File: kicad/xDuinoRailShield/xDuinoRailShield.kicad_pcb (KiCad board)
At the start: 2 copper layers, 63.5 x 53.3 mm, 40 parts, among them J501 Screw_Terminal_01x02, Q301 T2N7002BK, Q401 S8050, Q402 S8550, Q403 S8550, Q404 S8050, U201 TPS5430DDA, U301 6N137, U302 EL817

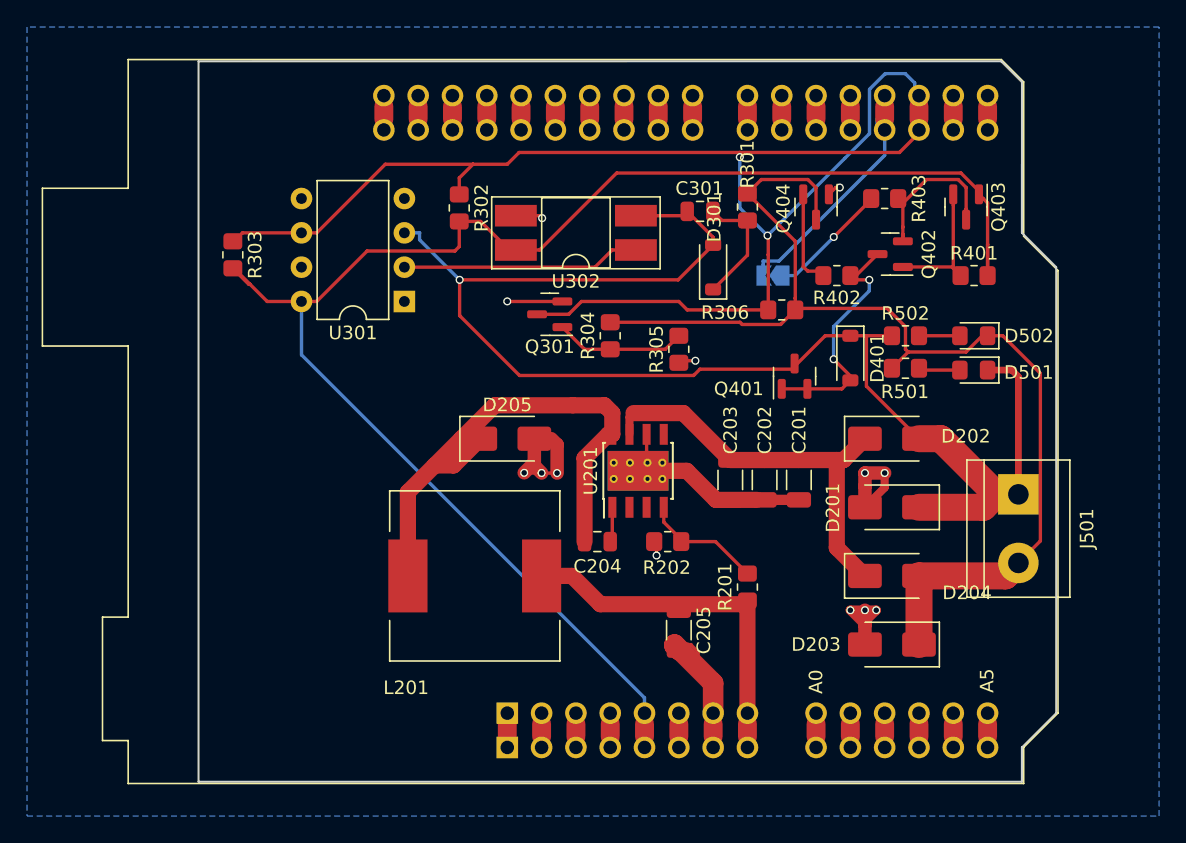
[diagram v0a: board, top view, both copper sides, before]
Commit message: xXiaoCentralMini
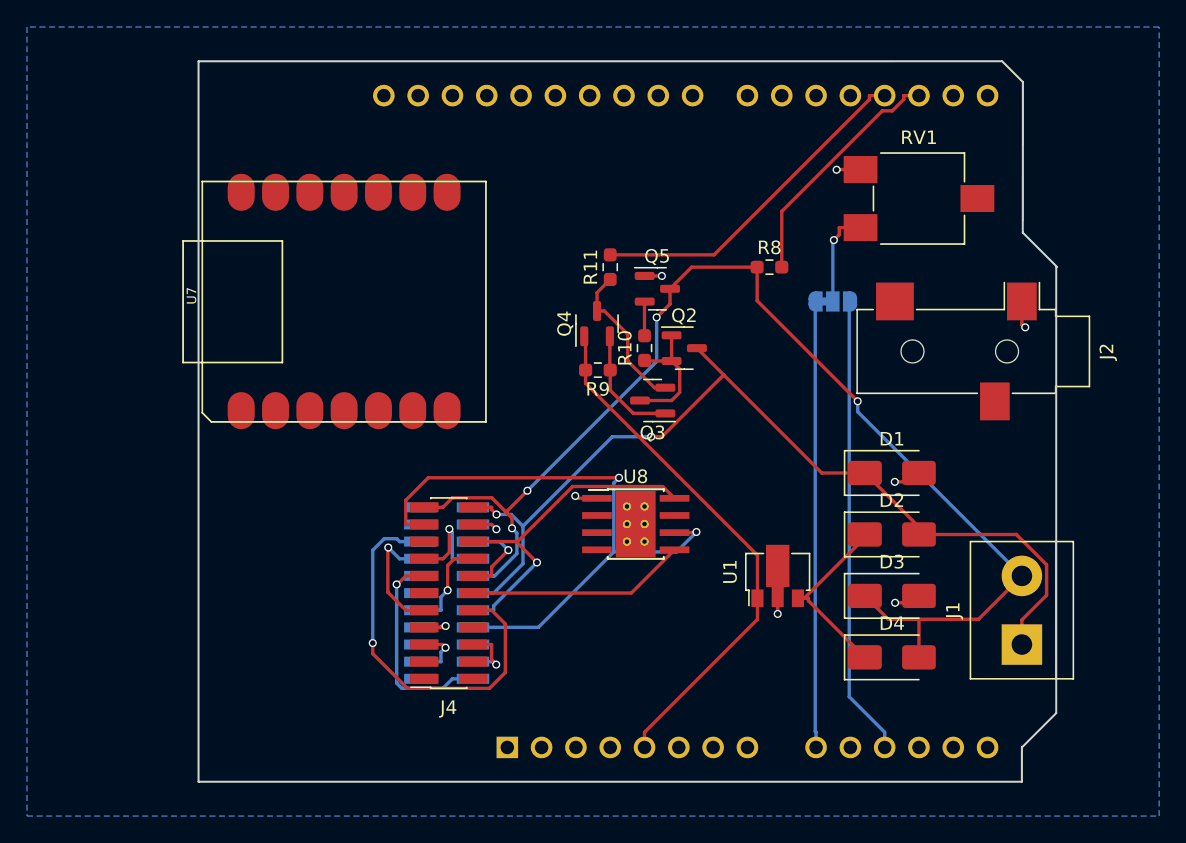
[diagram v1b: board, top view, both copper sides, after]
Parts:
- removed A501: Arduino_UNO_R3, Olis_Footprints:Arduino_UNO_R3_Double_Rows
- removed C201, C202, C203, C205: 10uF, Capacitor_SMD:C_1206_3216Metric
- removed C204: 10nF, Capacitor_SMD:C_0805_2012Metric
- removed C301: 1nF, Capacitor_SMD:C_0805_2012Metric
- removed D201, D202, D203, D204, D205: SS54, Diode_SMD:D_SMA
- removed D301, D401: 1N4148W, Diode_SMD:D_SOD-123
- removed D501, D502: LED, LED_SMD:LED_0805_2012Metric_Pad1.15x1.40mm_HandSolder
- removed J501: Screw_Terminal_01x02, TerminalBlock:TerminalBlock_bornier-2_P5.08mm
- removed JP_RAILCOM401: SolderJumper_2_Open, Jumper:SolderJumper-2_P1.3mm_Open_TrianglePad1.0x1.5mm
- removed L201: 22uH, Inductor_SMD:L_12x12mm_H8mm
- removed Q301: T2N7002BK, Package_TO_SOT_SMD:SOT-23
- removed Q401, Q404: S8050, Package_TO_SOT_SMD:SOT-23
- removed Q402, Q403: S8550, Package_TO_SOT_SMD:SOT-23
- removed R201, R403: 10k, Resistor_SMD:R_0805_2012Metric_Pad1.20x1.40mm_HandSolder
- removed R202: 1.58k, Resistor_SMD:R_0805_2012Metric_Pad1.20x1.40mm_HandSolder
- removed R301: 1k3, Resistor_SMD:R_0805_2012Metric_Pad1.20x1.40mm_HandSolder
- removed R302: 220R, Resistor_SMD:R_0805_2012Metric_Pad1.20x1.40mm_HandSolder
- removed R303: 5k, Resistor_SMD:R_0805_2012Metric_Pad1.20x1.40mm_HandSolder
- removed R304, R305, R402: 6k8, Resistor_SMD:R_0805_2012Metric_Pad1.20x1.40mm_HandSolder
- removed R306: 22k, Resistor_SMD:R_0805_2012Metric_Pad1.20x1.40mm_HandSolder
- removed R401: 20, Resistor_SMD:R_0805_2012Metric_Pad1.20x1.40mm_HandSolder
- removed R501, R502: 3k3, Resistor_SMD:R_0805_2012Metric_Pad1.20x1.40mm_HandSolder
- removed U201: TPS5430DDA, Package_SO:TI_SO-PowerPAD-8_ThermalVias
- removed U301: 6N137, Package_DIP:DIP-8_W7.62mm
- removed U302: EL817, Package_DIP:DIP-4_W8.89mm_SMDSocket_LongPads
- added A1: Arduino_UNO_R3, Module:Arduino_UNO_R3, B.Cu at (125.4, 92.4)
- added D1: SS54, Diode_SMD:D_SMA, F.Cu at (153.9, 72.1)
- added D2: SS54, Diode_SMD:D_SMA, F.Cu at (153.9, 76.6)
- added D3: SS54, Diode_SMD:D_SMA, F.Cu at (153.9, 81.2)
- added D4: SS54, Diode_SMD:D_SMA, F.Cu at (153.9, 85.7)
- added J1: Screw_Terminal_01x02, TerminalBlock:TerminalBlock_bornier-2_P5.08mm, F.Cu at (163.5, 84.8)
- added J2: AudioJack2_Ground, Connector_Audio:Jack_3.5mm_CUI_SJ-3523-SMT_Horizontal, F.Cu at (159.9, 63.1)
- added J3: PLUXX22, Connector_PinHeader_1.27mm:PinHeader_2x11_P1.27mm_Vertical_SMD, B.Cu at (120.9, 81.0)
- added J4: 21mtc, Connector_PinSocket_1.27mm:PinSocket_2x11_P1.27mm_Vertical_SMD, F.Cu at (121.1, 81.0)
- added JP1: DAC_OUTPUT_SELECT, Jumper:SolderJumper-3_P1.3mm_Bridged12_RoundedPad1.0x1.5mm, B.Cu at (149.5, 59.4)
- added Q2: S8050, Package_TO_SOT_SMD:SOT-23, F.Cu at (138.5, 62.8)
- added Q3: S8550, Package_TO_SOT_SMD:SOT-23, F.Cu at (136.2, 66.7)
- added Q4: S8550, Package_TO_SOT_SMD:SOT-23, F.Cu at (132.0, 61.0)
- added Q5: S8050, Package_TO_SOT_SMD:SOT-23, F.Cu at (136.5, 58.4)
- added R10: 6k8, Resistor_SMD:R_0603_1608Metric_Pad0.98x0.95mm_HandSolder, F.Cu at (135.6, 62.8)
- added R11: 10k, Resistor_SMD:R_0603_1608Metric_Pad0.98x0.95mm_HandSolder, F.Cu at (133.0, 56.8)
- added R8: 22k, Resistor_SMD:R_0603_1608Metric_Pad0.98x0.95mm_HandSolder, F.Cu at (144.8, 56.8)
- added R9: 20, Resistor_SMD:R_0603_1608Metric_Pad0.98x0.95mm_HandSolder, F.Cu at (132.1, 64.4)
- added RV1: 10K, Potentiometer_SMD:Potentiometer_ACP_CA6-VSMD_Vertical, F.Cu at (155.9, 51.7)
- added U1: L78L05_SOT89, Package_TO_SOT_SMD:SOT-89-3, F.Cu at (145.4, 79.4)
- added U7: MOUDLE-SEEEDUINO-XIAO-ESP32C3, xiao ESP32C3_PCB:MOUDLE14P-SMD-2.54-21X17.8MM, F.Cu at (123.8, 68.3)
- added U8: DRV8872DDA, Package_SO:Texas_HTSOP-8-1EP_3.9x4.9mm_P1.27mm_EP2.95x4.9mm_Mask2.4x3.1mm_ThermalVias, F.Cu at (134.9, 75.8)
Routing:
- net DCC_MM: track 113.1 -> 18.0 mm, vias 2 -> 0
- net +5V: track 117.9 -> 39.2 mm
- net GND: track 65.2 -> 14.6 mm, vias 13 -> 8
- net /Loco Adapters/MOTOR+: track 0.00 -> 46.4 mm, vias 0 -> 2
- net Net-(D205-K): track 39.0 -> 0.00 mm
- net /DCC1: track 106.5 -> 70.8 mm, vias 1 -> 2
- net /MCU Carrier Board/DAC_NUCLEO: track 0.00 -> 34.1 mm
- net /MCU Carrier Board/DAC_ADAFRUIT_SPARKFUN: track 0.00 -> 33.0 mm
- net /Loco Adapters/SPEAKER0: track 0.00 -> 29.4 mm, vias 0 -> 1
- net VCC: track 26.7 -> 0.00 mm
- net /Loco Adapters/MOTOR-: track 0.00 -> 25.5 mm, vias 0 -> 1
- net Net-(D401-A): track 18.0 -> 0.00 mm, vias 2 -> 0
- net DCC_0_1K3: track 17.0 -> 0.00 mm
- net DCC_VIN: track 30.4 -> 13.5 mm
- net /Loco Adapters/+5V: track 0.00 -> 16.3 mm
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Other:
- board size 63.5 x 53.3 mm -> 63.6 x 53.4 mm
